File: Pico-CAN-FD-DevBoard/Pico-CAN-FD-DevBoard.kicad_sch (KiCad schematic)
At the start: 53 parts, among them CN1 SM04B-SRSS-TB (LF)(SN), CN2 2601-1102, CN3 2601-1102, J1 Conn_01x03, J2 Conn_01x08, J3 USB_C_Receptacle_USB2.0_14P, SW1 SW_Push, SW2 SW_Push, U1 RP2350B, U2 MCP251863T-H-SS, U3 W25Q128JVS, U4 W25Q128JVS, U5 ESD2CAN24DBZRQ1, U6 TPS51386RJNR, Y1 ABM8-272-T3, Y2 Crystal 40MHz

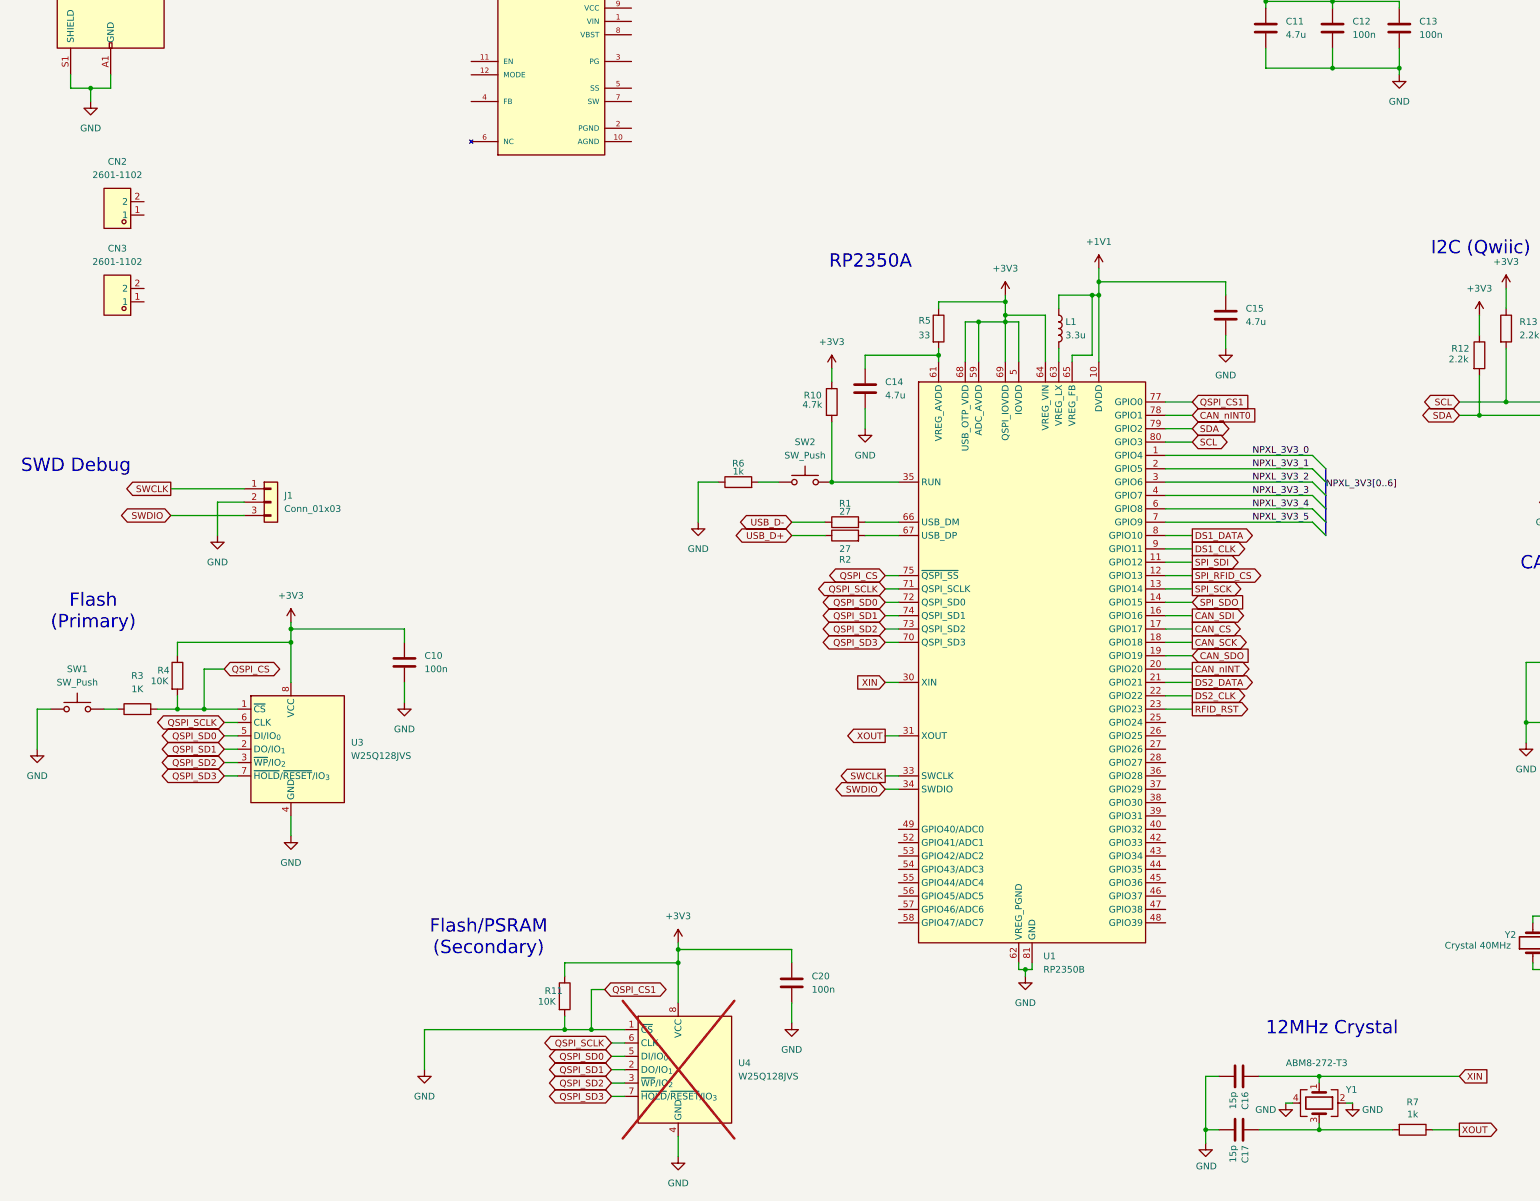
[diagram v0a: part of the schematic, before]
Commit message: fixed positions and typos
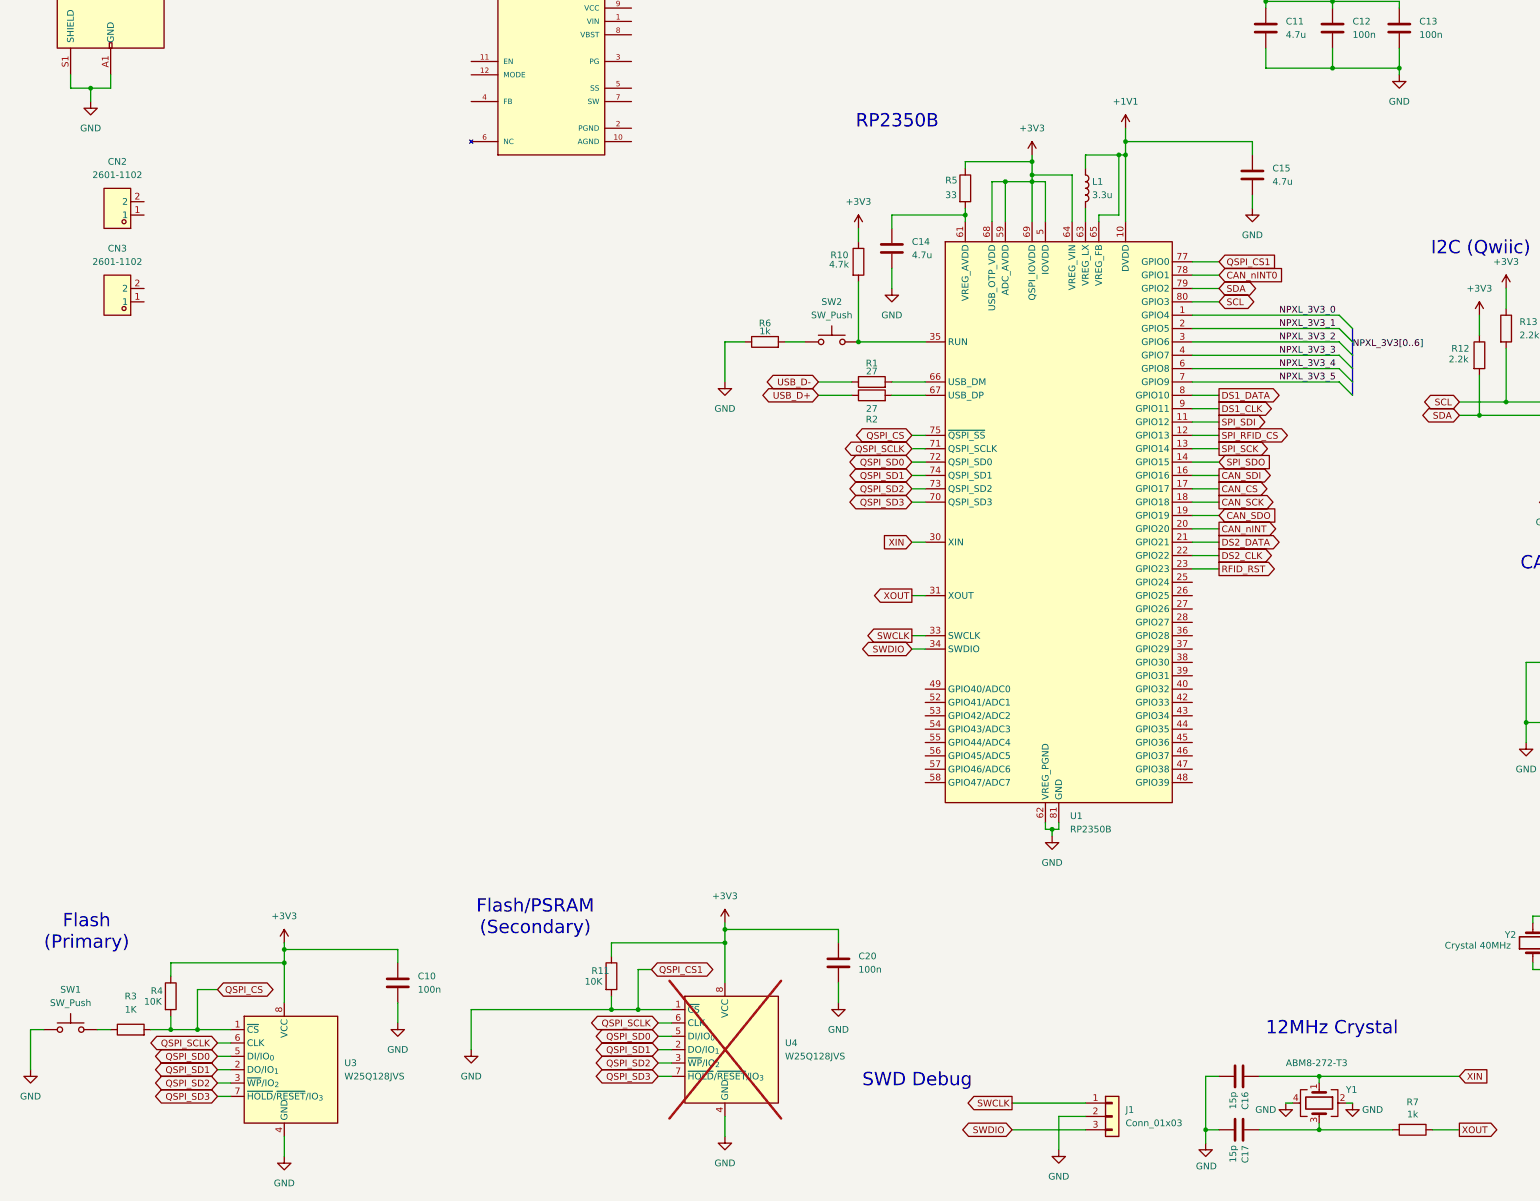
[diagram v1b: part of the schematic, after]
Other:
- note added: "RP2350B"
- note removed: "RP2350A"
- moved on the sheet: C10, C14, C15, C20, J1, L1, R1, R10, R11, R2, R3, R4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
